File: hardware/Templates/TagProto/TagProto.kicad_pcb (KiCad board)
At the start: 2 copper layers, 20 parts, among them J201 CONN_02X04, J401 CONN_01X02, Q501 Q_NPN_BEC, U1 at25ff321D-UUN, U302 stm32l431kc, U501 RV-3028-C7

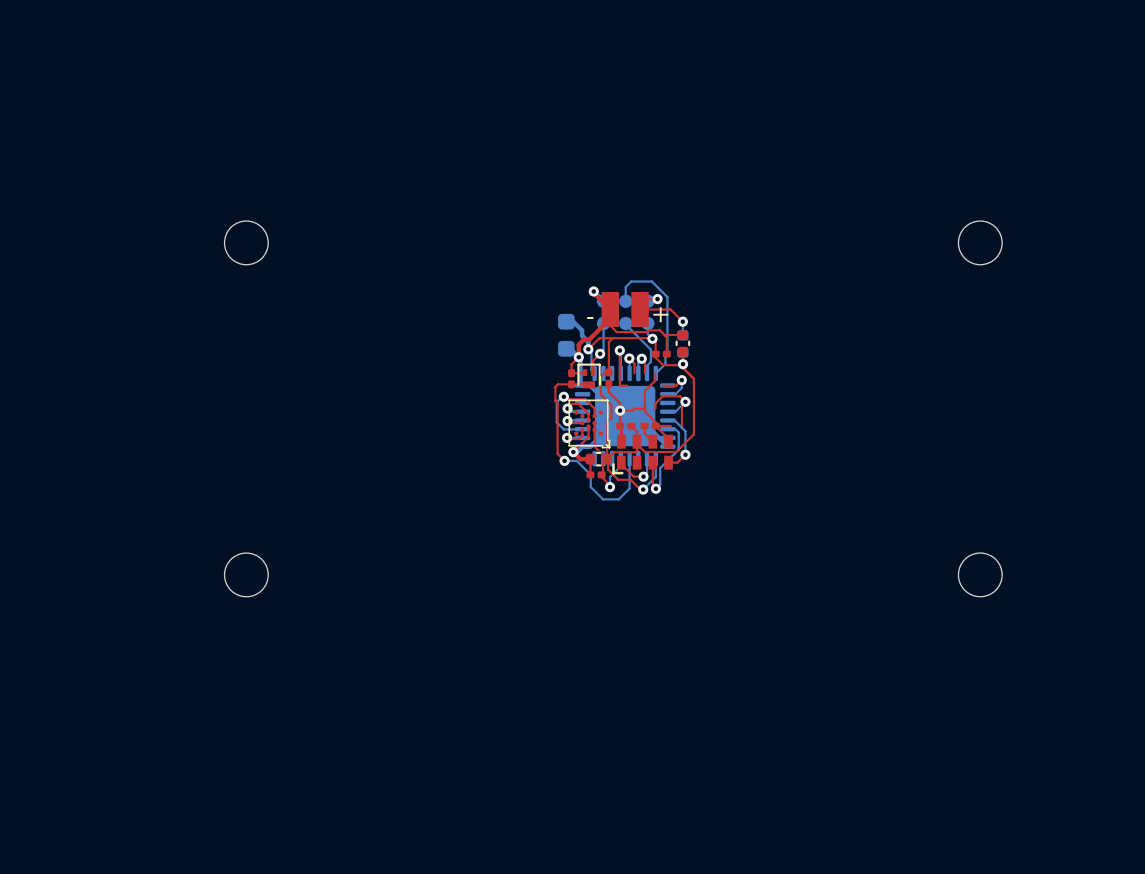
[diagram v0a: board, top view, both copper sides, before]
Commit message: checkpoint
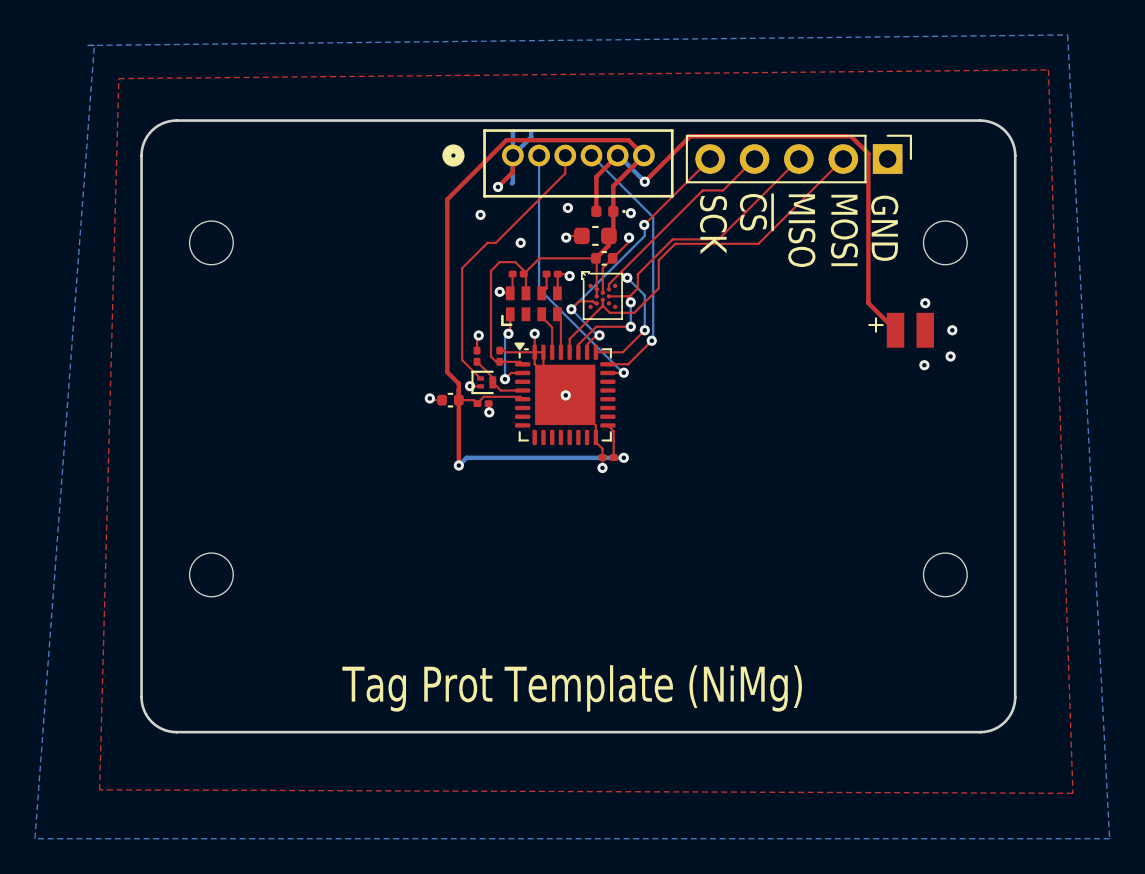
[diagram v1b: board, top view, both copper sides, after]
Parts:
- removed J201: CONN_02X04, bittag:tagpoints6
- added J1: Conn_01x06, library:CONN_B6B-ZR_JST, F.Cu at (121.2, 87.0)
- added J2: Conn_01x04, Connector_PinHeader_2.54mm:PinHeader_1x05_P2.54mm_Vertical, F.Cu at (142.7, 87.2)
- C4, D401, U302: moved to F.Cu
- J401: footprint bittag:MS621 -> library:MS621
- moved J401 16.4 mm to (144.0, 97.0), turned to 90 degrees
- moved C3 13.7 mm to (117.7, 101.0), turned to 180 degrees
- moved C404 11.5 mm to (126.5, 92.9), turned to 0 degrees
- moved C503 10.6 mm to (121.6, 93.8)
- moved U501 10.6 mm to (122.5, 95.5)
- moved C501 10.6 mm to (119.5, 101.2)
- moved R1 10.3 mm to (123.5, 93.8)
- moved D401 8.80 mm to (126.5, 90.2), turned to 180 degrees
- moved U1 7.30 mm to (126.4, 95.1), turned to 0 degrees
- moved C101 6.37 mm to (120.5, 98.5), turned to 90 degrees
- moved C4 5.92 mm to (126.0, 91.6), turned to 180 degrees
- moved Q501 5.86 mm to (119.8, 100.0), turned to 0 degrees
- moved C502 5.56 mm to (119.2, 98.5)
- moved U302 3.64 mm to (124.2, 100.7), turned to 0 degrees
- moved H1 2.00 mm to (104.0, 92.0)
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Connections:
- net /SCL renamed /RTC_SCL
- net /SDA renamed /RTC_SDA
- U302 pad 10: /AT25_nCS -> /PA4
- U302 pad 11: /AT25_SCK -> /PA5_SCK
- U302 pad 12: /AT25_MISO -> /PA6_MISO
- U302 pad 13: /AT25_MOSI -> /PA7_MOSI
- U302 pad 14: unconnected-(U302-PB0-Pad14) -> /PB0
- U302 pad 15: unconnected-(U302-PB1-Pad15) -> /PB1
- U302 pad 18: unconnected-(U302-PA8-Pad18) -> /PA8
- U302 pad 19: unconnected-(U302-PA9-Pad19) -> /PA9
- U302 pad 20: unconnected-(U302-PA10-Pad20) -> /PA10
- U302 pad 21: unconnected-(U302-PA11-Pad21) -> /PA11_MISO
- U302 pad 22: unconnected-(U302-PA12-Pad22) -> /PA12_MOSI
- U302 pad 25: unconnected-(U302-PA15-Pad25) -> /AT25_nCS
- U302 pad 26: unconnected-(U302-PB3-Pad26) -> /AT25_SCK
- U302 pad 27: unconnected-(U302-PB4-Pad27) -> /AT25_MISO
- U302 pad 28: unconnected-(U302-PB5-Pad28) -> /AT25_MOSI
- U302 pad 6: unconnected-(U302-PA0-Pad6) -> /PA0
- U302 pad 7: unconnected-(U302-PA1-Pad7) -> /PA1_SCK
- U302 pad 8: unconnected-(U302-PA2-Pad8) -> /PA2
- U302 pad 9: unconnected-(U302-PA3-Pad9) -> /PA3
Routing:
- net VBAT: track 5.55 -> 30.9 mm, vias 2 -> 1
- net VIN: track 44.4 -> 69.6 mm, vias 5 -> 2
- net /AT25_MOSI: track 3.49 -> 22.3 mm, vias 1 -> 0
- net /AT25_MISO: track 1.78 -> 20.3 mm, vias 1 -> 2
- net /AT25_nCS: track 2.26 -> 18.8 mm, vias 1 -> 2
- net RST: track 3.07 -> 15.9 mm, vias 1 -> 0
- net SWDIO: track 3.55 -> 15.4 mm, vias 0 -> 1
- net GND: track 51.1 -> 39.9 mm, vias 4 -> 20
- net /AT25_SCK: track 6.20 -> 17.3 mm, vias 1 -> 3
- net Net-(Q501-C): track 13.5 -> 3.46 mm, vias 1 -> 0
- net SWCLK: track 8.35 -> 15.2 mm, vias 0 -> 1
- net unconnected-(U302-PB5-Pad28): track 5.03 -> 0.00 mm, vias 1 -> 0
- net unconnected-(U302-PA10-Pad20): track 3.75 -> 0.00 mm, vias 1 -> 0
- net /RTC_SCL: track 5.74 -> 2.42 mm, vias 1 -> 0
- net unconnected-(U302-PB3-Pad26): track 3.00 -> 0.00 mm, vias 1 -> 0
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- added copper zone on B.Cu, net GND
- added copper zone on F.Cu, net GND
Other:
- board outline added: 50 x 35 mm
- board text added: "GND"
- board text added: "MISO"
- board text added: "MOSI"
- board text added: "SCK"
- board text added: "Tag Prot Template (NiMg)"
- board text added: "~{CS}"
